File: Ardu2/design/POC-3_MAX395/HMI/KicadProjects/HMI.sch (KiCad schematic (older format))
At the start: 13 parts

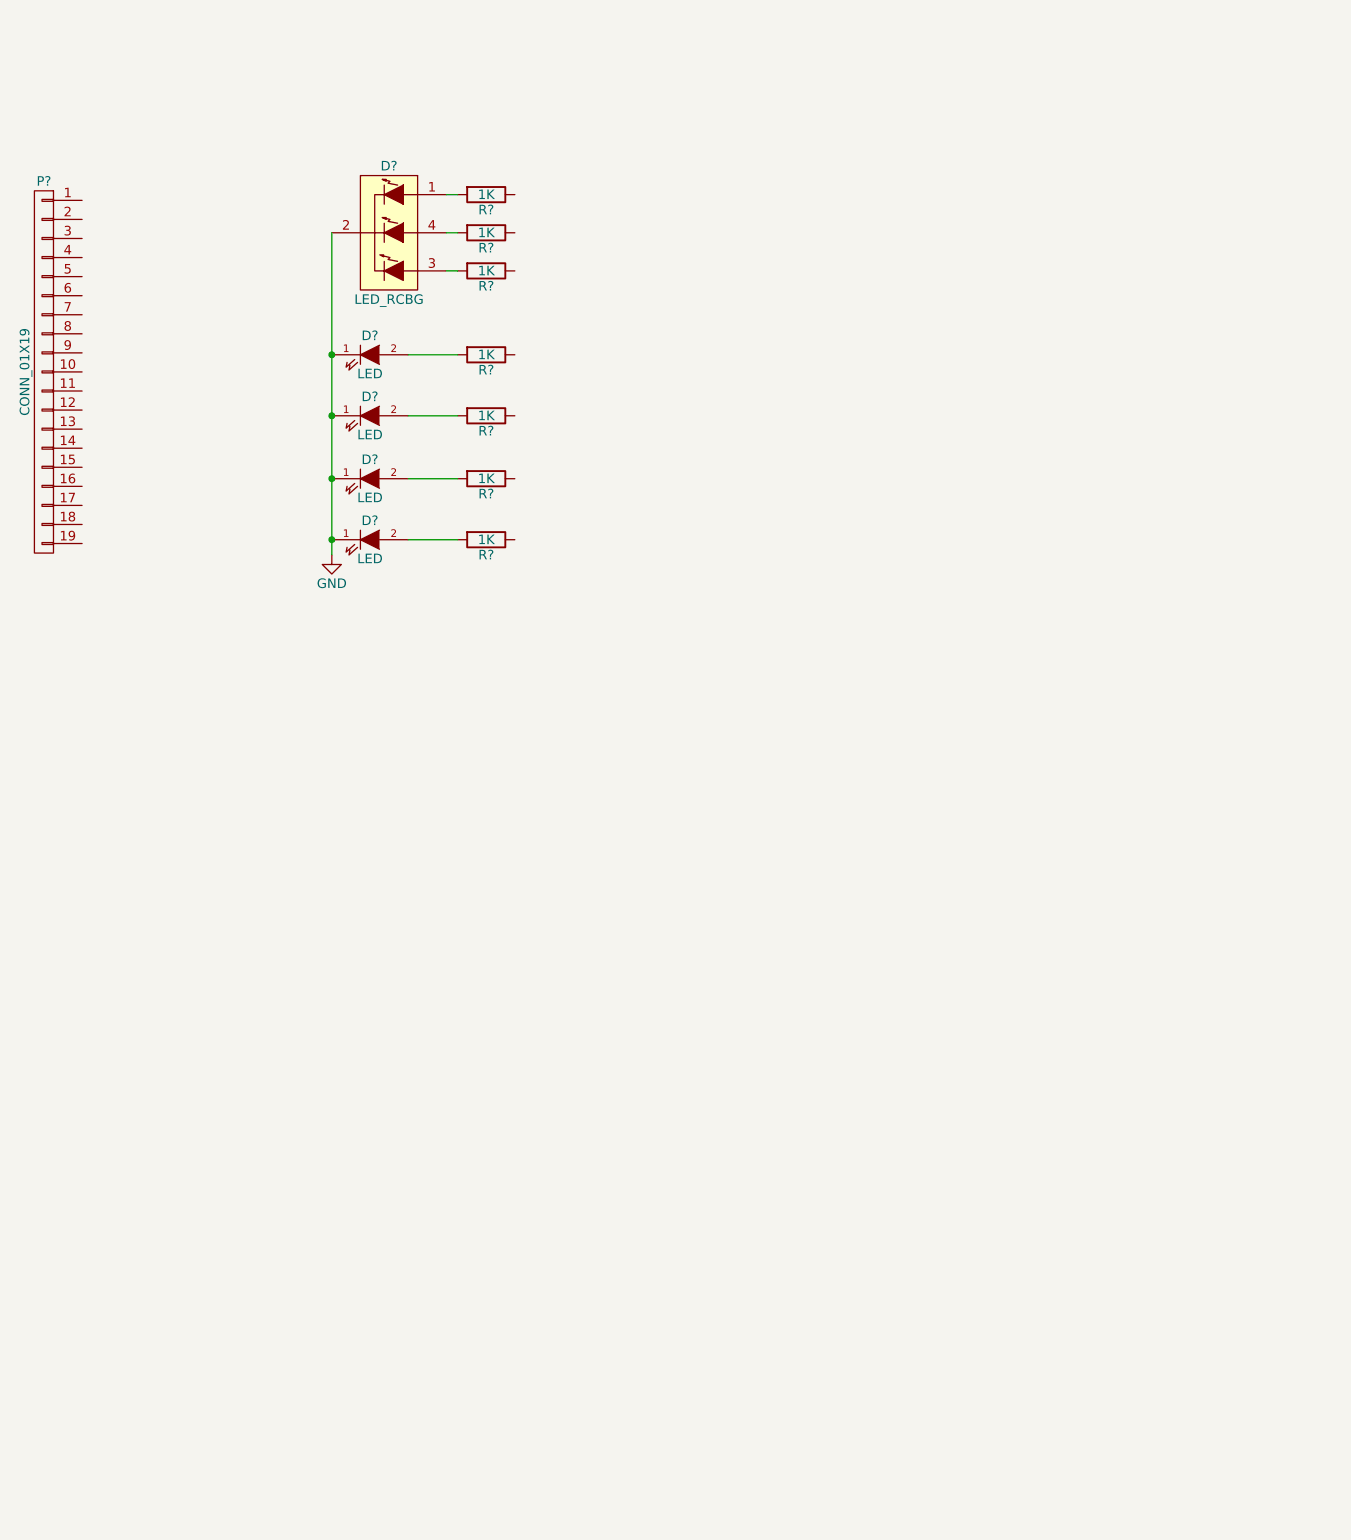
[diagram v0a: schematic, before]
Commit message: HMI LED PCB 00
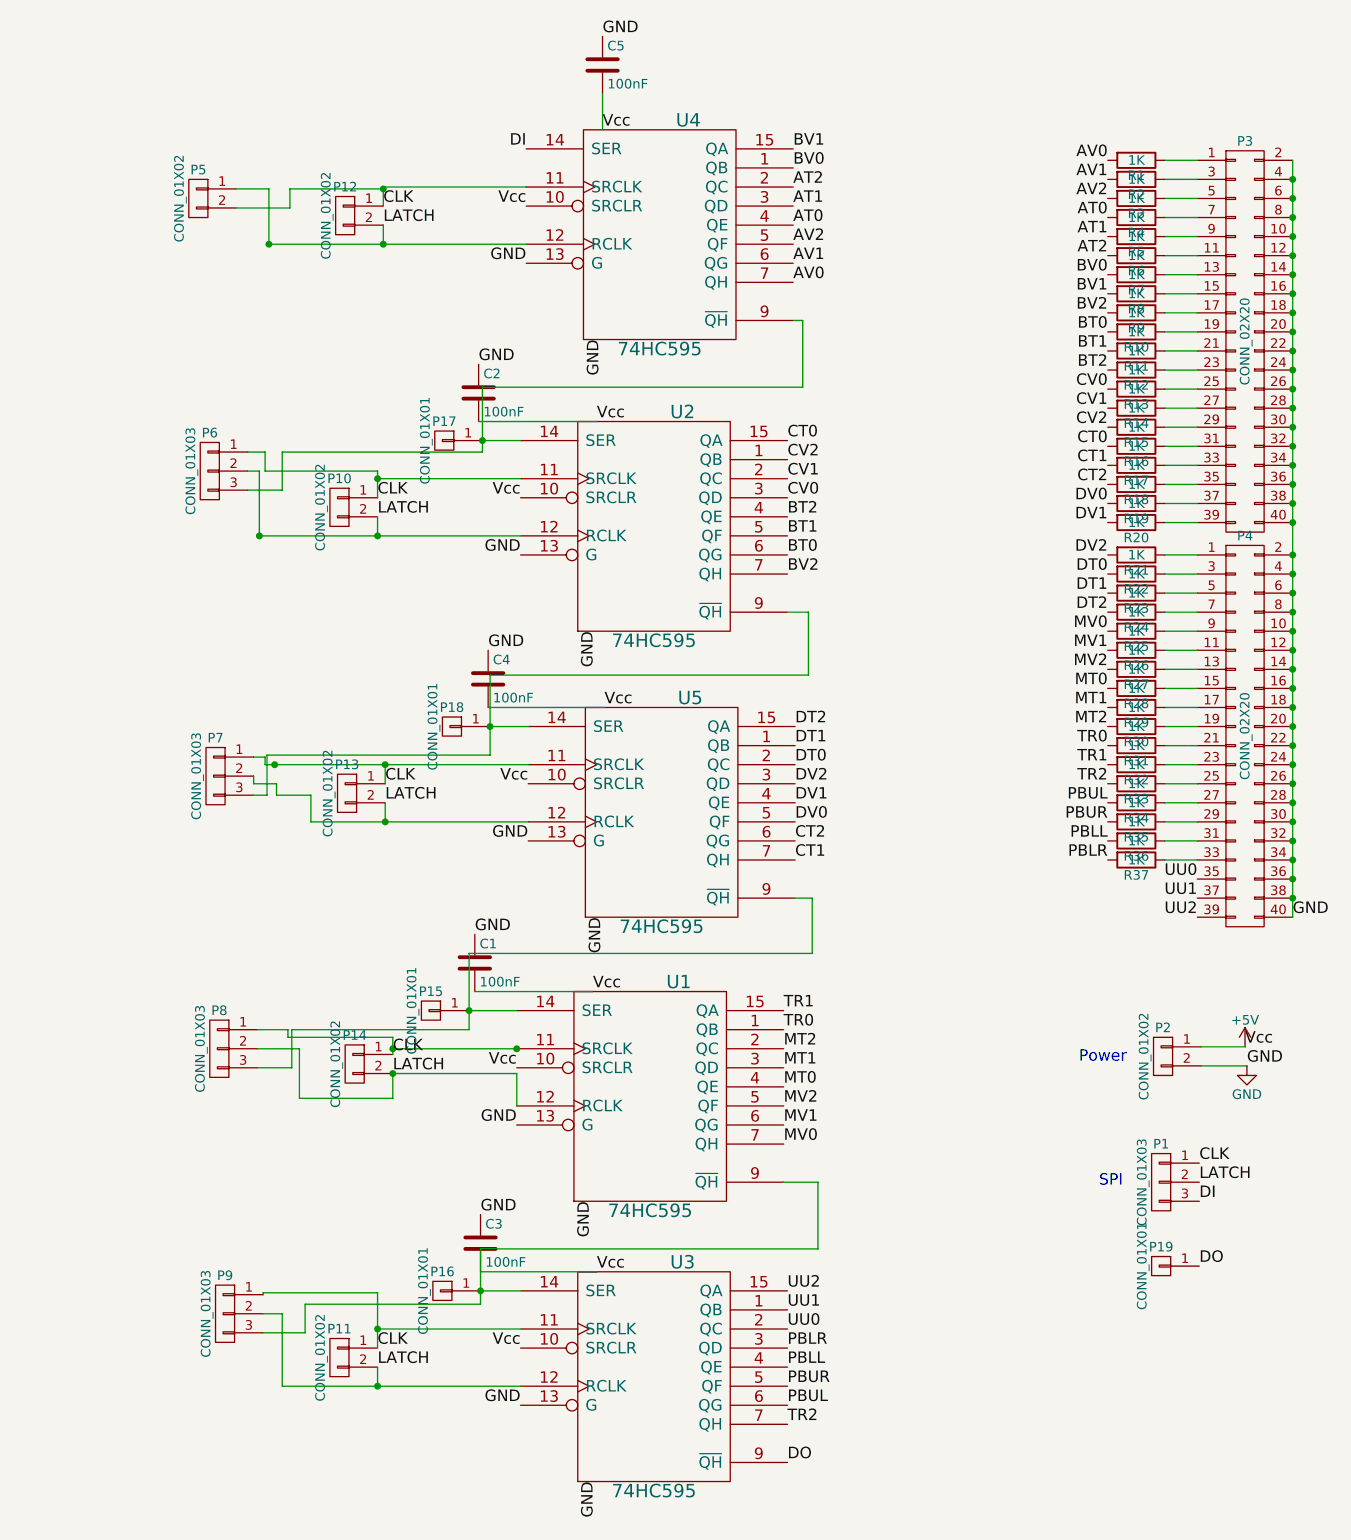
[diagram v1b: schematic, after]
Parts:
- removed D? (x4): LED, symbol LED
- removed D?: LED_RCBG, symbol LED_RCBG
- removed P?: CONN_01X19, symbol CONN_01X19
- removed R? (x7): 1K, symbol R
- added C1, C2, C3, C4, C5: 100nF, Capacitors_ThroughHole:C_Disc_D3_P2.5, symbol C
- added P1, P6, P7, P8, P9: CONN_01X03, Pin_Headers:Pin_Header_Straight_1x03, symbol CONN_01X03
- added P10, P11, P12, P13, P14, P2, P5: CONN_01X02, Pin_Headers:Pin_Header_Straight_1x02, symbol CONN_01X02
- added P15, P16, P17, P18, P19: CONN_01X01, Pin_Headers:Pin_Header_Straight_1x01, symbol CONN_01X01
- added P3, P4: CONN_02X20, Pin_Headers:Pin_Header_Straight_2x20, symbol CONN_02X20
- added R1, R10, R11, R12, R13, R14, R15, R16, R17, R18, R19, R2, R20, R21, R22, R23, R24, R25, R26, R27, R28, R29, R3, R30, R31, R32, R33, R34, R35, R36, R37, R4, R5, R6, R7, R8, R9: 1K, Resistors_ThroughHole:Resistor_Horizontal_RM10mm, symbol R
- added U1, U2, U3, U4, U5: 74HC595, Housings_DIP:DIP-16_W7.62mm, symbol 74HC595
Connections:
- net labels added: +5V, AT0, AT1, AT2, AV0, AV1, AV2, BT0, BT1, BT2, BV0, BV1, BV2, CLK, CT0, CT1, CT2, CV0, CV1, CV2, DI, DO, DT0, DT1, DT2, DV0, DV1, DV2, LATCH, MT0, MT1, MT2, MV0, MV1, MV2, PBLL, PBLR, PBUL, PBUR, TR0, TR1, TR2, UU0, UU1, UU2, Vcc
- wire segments 9 -> 126
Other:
- note added: "Power"
- note added: "SPI"

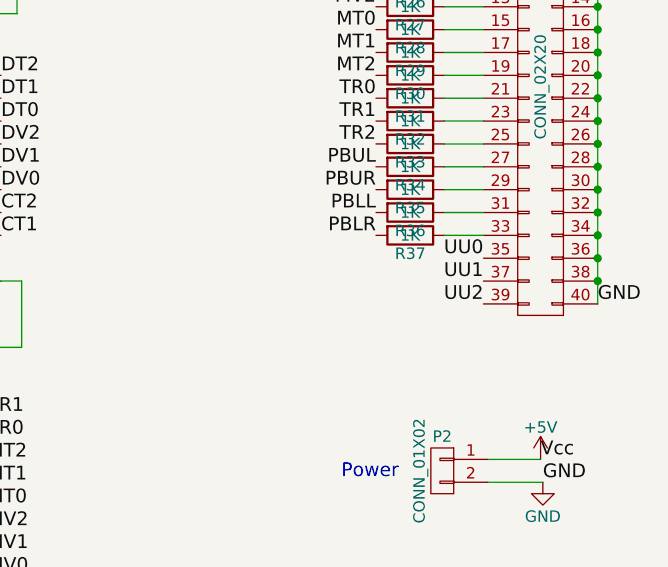
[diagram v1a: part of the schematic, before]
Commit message: HMI PCB v2a
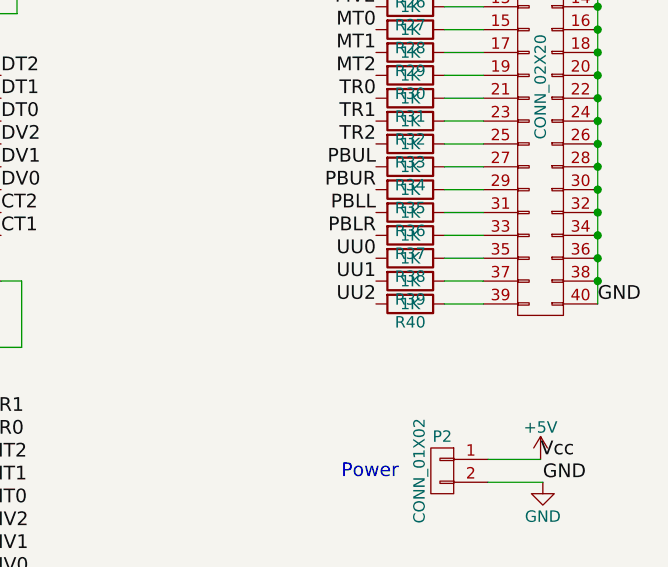
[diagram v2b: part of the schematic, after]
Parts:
- added R38, R39, R40: 1K, Resistors_ThroughHole:Resistor_Horizontal_RM10mm, symbol R
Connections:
- net UU0: now also R38.2; no longer P4.35 (P35)
- net UU1: now also R39.2; no longer P4.37 (P37)
- net UU2: now also R40.2; no longer P4.39 (P39)
- new net: P4.35 (P35), R38.1
- new net: P4.37 (P37), R39.1
- new net: P4.39 (P39), R40.1
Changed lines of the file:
@@
 Sheet 1 1
 Title "PyGuitar HMI LED Circuit"
-Date "2015-11-17"
-Rev "0"
-Comp ""
-Comment1 ""
+Date "2015-11-18"
+Rev "1"
+Comp "Gratefulfrog"
+Comment1 "added 3 resistors to complete circuit!"
 Comment2 ""
 Comment3 ""
@@
 Text Label 7210 4970 2    60   ~ 0
 TR2
-Text Label 7680 5470 2    60   ~ 0
+Text Label 7210 5470 2    60   ~ 0
 UU0
-Text Label 7680 5570 2    60   ~ 0
+Text Label 7210 5570 2    60   ~ 0
 UU1
-Text Label 7680 5670 2    60   ~ 0
+Text Label 7210 5670 2    60   ~ 0
 UU2
 Text Label 7210 5370 2    60   ~ 0
@@
 	-1   0    0    -1
 $EndComp
+$Comp
+L R R38
+U 1 1 564C39C7
+P 7360 5470
+F 0 "R38" V 7440 5470 50  0000 C CNN
+F 1 "1K" V 7360 5470 50  0000 C CNN
+F 2 "Resistors_ThroughHole:Resistor_Horizontal_RM10mm" V 7290 5470 30  0001 C CNN
+F 3 "" H 7360 5470 30  0000 C CNN
+	1    7360 5470
+	0    1    1    0
+$EndComp
+$Comp
+L R R39
+U 1 1 564C3B87
+P 7360 5570
+F 0 "R39" V 7440 5570 50  0000 C CNN
+F 1 "1K" V 7360 5570 50  0000 C CNN
+F 2 "Resistors_ThroughHole:Resistor_Horizontal_RM10mm" V 7290 5570 30  0001 C CNN
+F 3 "" H 7360 5570 30  0000 C CNN
+	1    7360 5570
+	0    1    1    0
+$EndComp
+$Comp
+L R R40
+U 1 1 564C3C8B
+P 7360 5670
+F 0 "R40" V 7440 5670 50  0000 C CNN
+F 1 "1K" V 7360 5670 50  0000 C CNN
+F 2 "Resistors_ThroughHole:Resistor_Horizontal_RM10mm" V 7290 5670 30  0001 C CNN
+F 3 "" H 7360 5670 30  0000 C CNN
+	1    7360 5670
+	0    1    1    0
+$EndComp
+Wire Wire Line
+	7510 5470 7680 5470
+Wire Wire Line
+	7680 5570 7510 5570
+Wire Wire Line
+	7510 5670 7680 5670
 $EndSCHEMATC
